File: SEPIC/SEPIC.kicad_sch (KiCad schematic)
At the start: 9 parts, among them Q1 NMOS

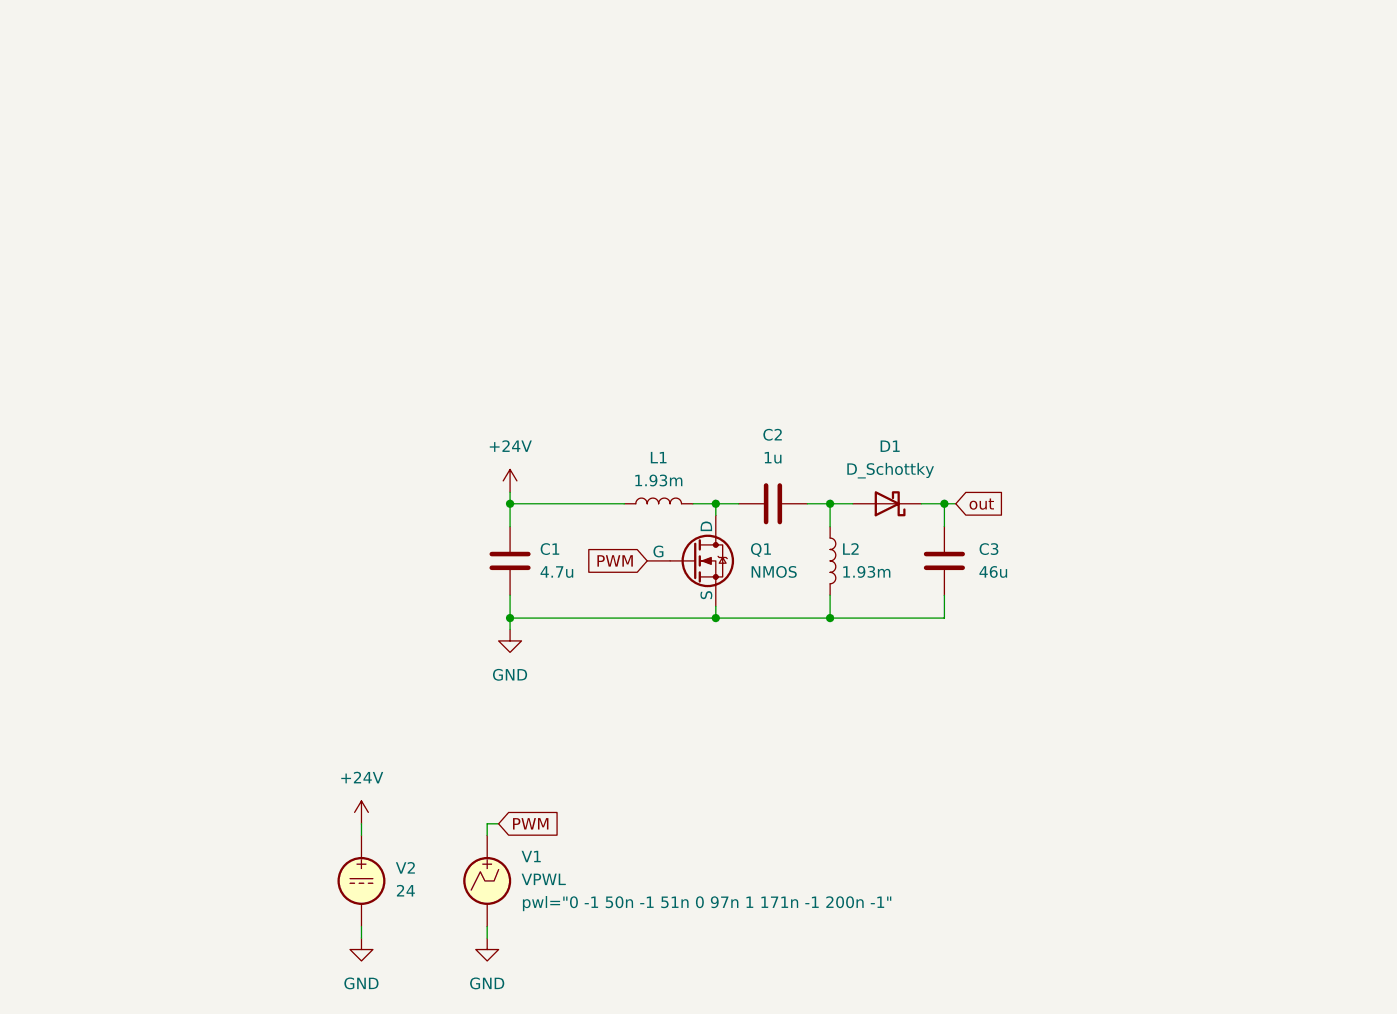
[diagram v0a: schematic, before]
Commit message: Placa v0.1
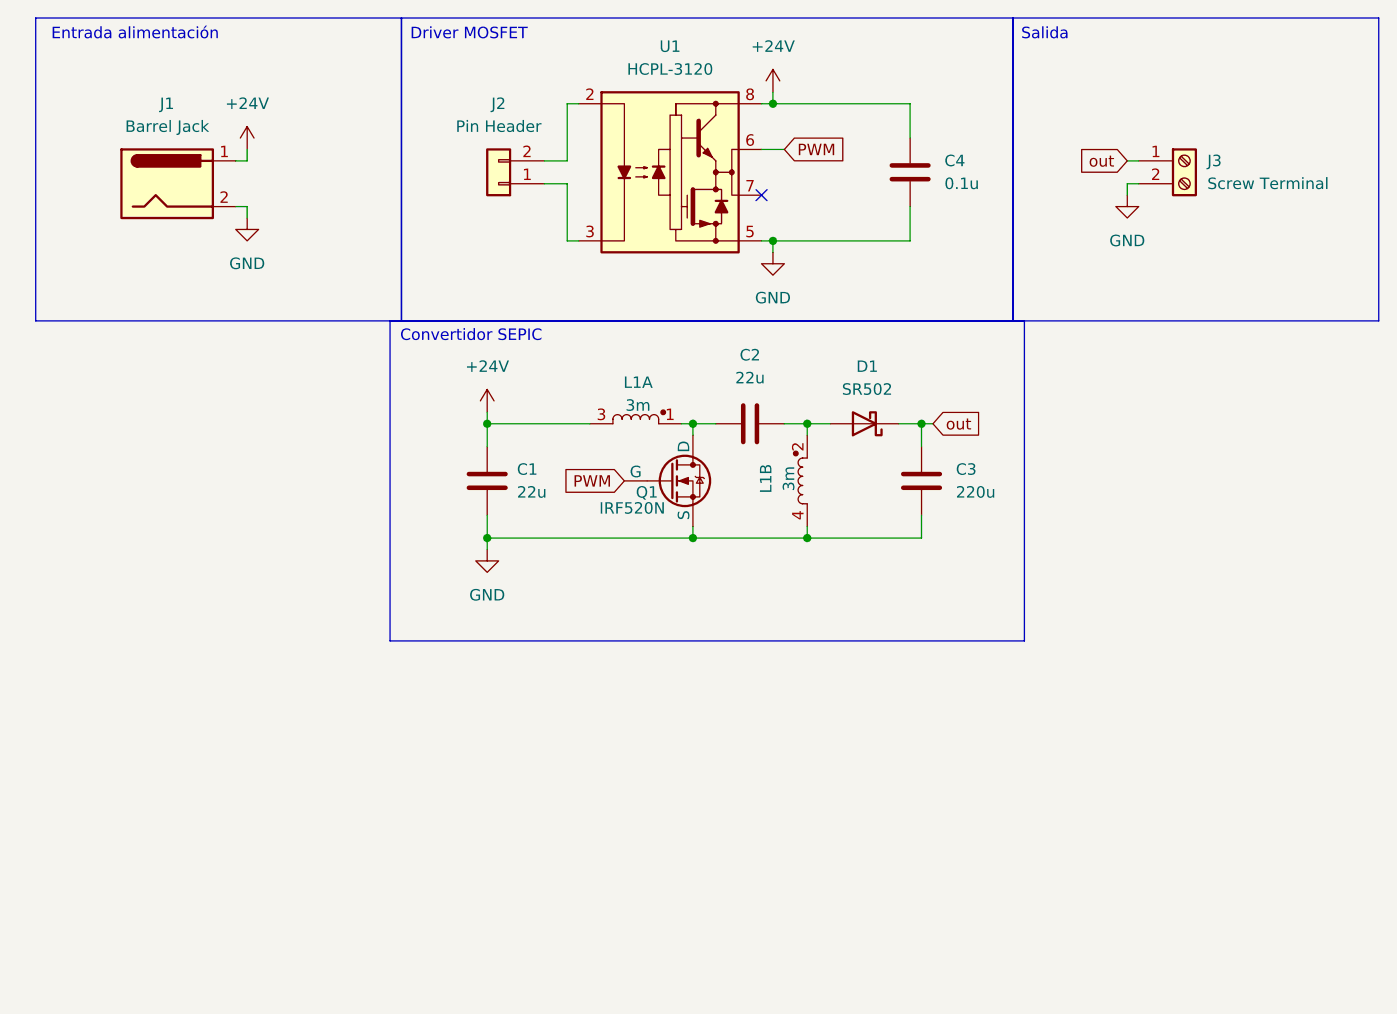
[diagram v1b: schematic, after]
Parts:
- removed L2: 1.93m, symbol Device:L
- removed V1: VPWL, symbol Simulation_SPICE:VPWL
- removed V2: 24, symbol Simulation_SPICE:VDC
- added C4: 0.1u, Capacitor_THT:C_Disc_D3.8mm_W2.6mm_P2.50mm, symbol Device:C
- added J1: Barrel Jack, Connector_BarrelJack:BarrelJack_Horizontal, symbol Connector:Barrel_Jack
- added J2: Pin Header, Connector_PinHeader_2.54mm:PinHeader_1x02_P2.54mm_Horizontal, symbol Connector_Generic:Conn_01x02
- added J3: Screw Terminal, TerminalBlock_Phoenix:TerminalBlock_Phoenix_MKDS-1,5-2-5.08_1x02_P5.08mm_Horizontal, symbol Connector:Screw_Terminal_01x02
- added U1: HCPL-3120, Package_DIP:DIP-8_W7.62mm, symbol Driver_FET:HCPL-3120
- C1: value 4.7u -> 22u; footprint (none) -> Capacitor_THT:C_Radial_D4.0mm_H7.0mm_P1.50mm
- C2: value 1u -> 22u; footprint (none) -> Capacitor_THT:C_Radial_D4.0mm_H7.0mm_P1.50mm
- C3: value 46u -> 220u; footprint (none) -> Capacitor_THT:C_Radial_D10.0mm_H16.0mm_P5.00mm
- D1: value D_Schottky -> SR502; footprint (none) -> Diode_THT:D_A-405_P7.62mm_Horizontal
- L1: value 1.93m -> 3m; footprint (none) -> Inductor_THT:L_CommonMode_Toroid_Vertical_L43.2mm_W22.9mm_Px17.78mm_Py30.48mm_Bourns_8100; symbol Device:L -> Inductor:L_Coupled
- Q1: value NMOS -> IRF520N; footprint (none) -> Package_TO_SOT_THT:TO-3P-3_Vertical
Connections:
- net +24V: now also L1.3, C4.1, J1.1, U1.8 (VCC); no longer L1.1
- net GND: now also L1.4, C4.2, J1.2, J3.2 (Pin_2), U1.5 (VEE)
- net PWM: now also U1.6 (VO)
- net out: now also J3.1 (Pin_1)
- net at C2.2, D1.2 (A): now also L1.2
- net at C2.1, Q1.1 (D): now also L1.1; no longer L1.2
- new net: J2.1 (Pin_1), U1.3 (C)
- new net: J2.2 (Pin_2), U1.2 (A)
- no-connect marks 0 -> 1
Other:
- note added: "Convertidor SEPIC"
- note added: "Driver MOSFET"
- note added: "Entrada alimentación"
- note added: "Salida"
- company: (none) -> Universidad de Concepción
- title: (none) -> Convertidor DC/DC Sepic
- moved on the sheet: C1, C2, C3, D1, Q1
